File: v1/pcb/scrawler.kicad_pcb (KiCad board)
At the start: 2 copper layers, 185.3 x 172.6 mm, 97 parts, among them J2 MJ-4PP-9, J3 OLED, SW10A1 SW_PUSH, SW10B1 SW_PUSH, SW11A1 SW_PUSH, SW11B1 SW_PUSH, SW12A1 SW_PUSH, SW12B1 SW_PUSH, SW13A1 SW_PUSH, SW13B1 SW_PUSH, SW14A1 SW_PUSH, SW14B1 SW_PUSH, SW15A1 SW_PUSH, SW15B1 SW_PUSH, SW16A1 SW_PUSH, SW16B1 SW_PUSH, SW17A1 SW_PUSH, SW17B1 SW_PUSH, SW18A1 SW_PUSH, SW18B1 SW_PUSH, SW19A1 SW_PUSH, SW19B1 SW_PUSH, SW1A1 SW_PUSH, SW1B1 SW_PUSH, SW20A1 SW_PUSH, SW20B1 SW_PUSH, SW21A1 SW_PUSH, SW21B1 SW_PUSH, SW22A1 SW_PUSH, SW22B1 SW_PUSH, SW24A1 SW_PUSH, SW24B1 SW_PUSH, SW25A1 SW_PUSH, SW25B1 SW_PUSH, SW26 Rotary_Encoder_Switch, SW26A1 SW_PUSH, SW26B1 SW_PUSH, SW2A1 SW_PUSH, SW2B1 SW_PUSH, SW3A1 SW_PUSH, SW3B1 SW_PUSH, SW4A1 SW_PUSH, SW4B1 SW_PUSH, SW5A1 SW_PUSH, SW5B1 SW_PUSH, SW6A1 SW_PUSH, SW6B1 SW_PUSH, SW7A1 SW_PUSH, SW7B1 SW_PUSH, SW8A1 SW_PUSH, SW8B1 SW_PUSH, SW9A1 SW_PUSH, SW9B1 SW_PUSH, U1 ProMicro

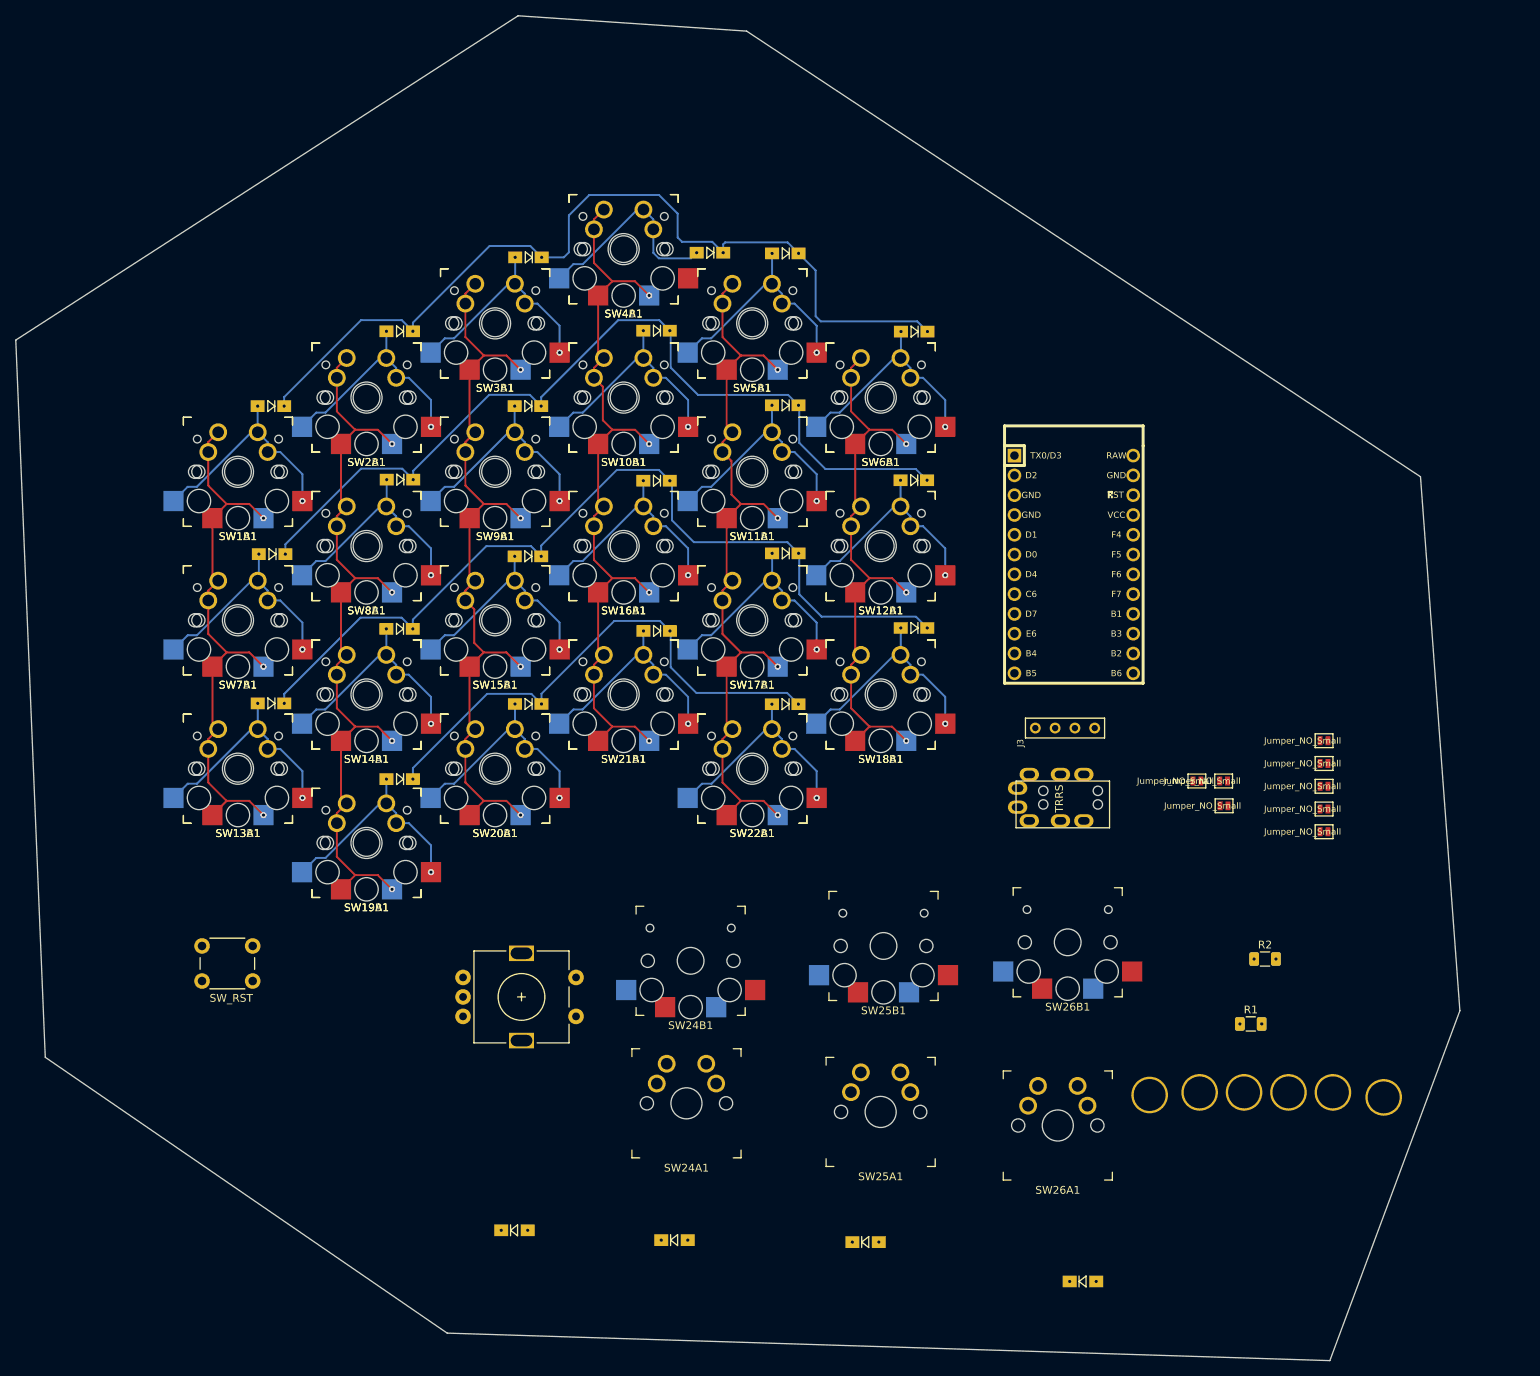
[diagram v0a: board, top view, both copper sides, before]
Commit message: pcb done
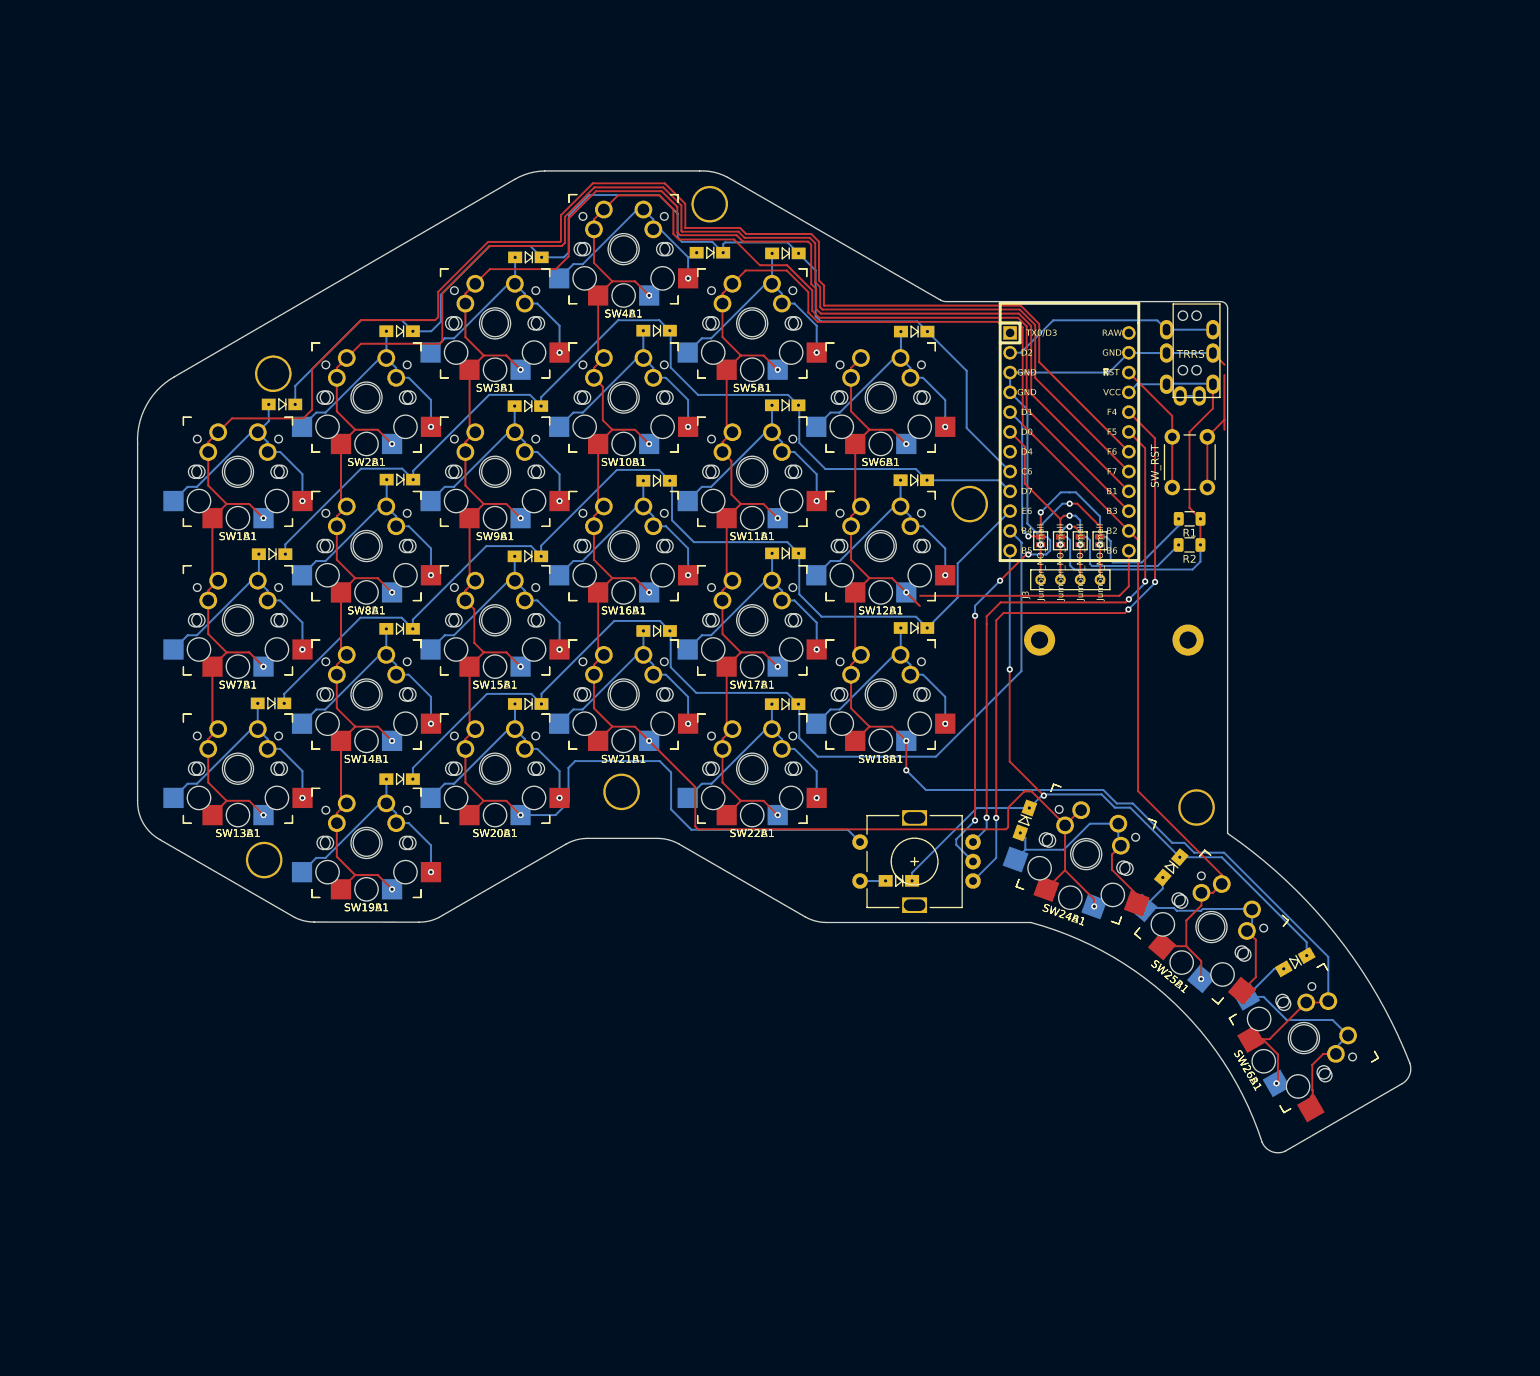
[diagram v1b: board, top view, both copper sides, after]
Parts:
- added H7: Hole, SofleKeyboard-footprint:M2_HOLE_PCB, F.Cu at (179.1, 97.8)
- added H8: Hole, SofleKeyboard-footprint:M2_HOLE_PCB, F.Cu at (198.1, 97.8)
- JP5, JP6, JP7, JP8: moved to B.Cu
- moved H1 145.6 mm to (80.7, 63.6)
- moved RSW1 144.6 mm to (200.6, 71.7), turned to 270 degrees
- moved H6 143.6 mm to (136.7, 41.9)
- moved H2 123.7 mm to (79.6, 126.0)
- moved H5 88.7 mm to (170.1, 80.3)
- moved H3 88.7 mm to (125.4, 117.3)
- moved D24 70.1 mm to (177.2, 120.9), turned to 250 degrees
- moved D23 66.7 mm to (161.0, 128.7), turned to 180 degrees
- moved R1 65.3 mm to (198.3, 82.2), turned to 180 degrees
- moved J2 65.2 mm to (199.2, 54.7), turned to 0 degrees
- moved D25 62.1 mm to (196.0, 127.0), turned to 230 degrees
- moved SW24A1 60.4 mm to (185.1, 125.3), turned to 340 degrees
- moved R2 54.0 mm to (198.3, 85.6), turned to 180 degrees
- moved SW26 53.4 mm to (163.0, 126.2), turned to 180 degrees
- moved SW24B1 52.6 mm to (185.1, 125.3), turned to 340 degrees
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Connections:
- SW24A1 pad 1: COL1 -> COL3
- SW24B1 pad 1: COL1 -> COL3
- SW25A1 pad 1: COL2 -> COL4
- SW25B1 pad 1: COL2 -> COL4
- SW26 pad S1: COL0 -> COL2
- SW26A1 pad 1: COL3 -> COL5
- SW26B1 pad 1: COL3 -> COL5
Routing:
- net COL3: track 100.1 -> 279.2 mm, vias 4 -> 5
- net COL2: track 100.1 -> 275.2 mm
- net COL0: track 75.5 -> 235.9 mm
- net COL4: track 100.1 -> 243.4 mm, vias 4 -> 5
- net COL1: track 102.8 -> 243.2 mm
- net GND: track 0.00 -> 131.5 mm, vias 0 -> 5
- net COL5: track 73.0 -> 199.3 mm, vias 3 -> 5
- net ROW4: track 0.00 -> 98.9 mm, vias 0 -> 2
- net ENCA: track 0.00 -> 80.4 mm, vias 0 -> 3
- net ENCB: track 0.00 -> 72.1 mm, vias 0 -> 3
- net VCC: track 0.00 -> 62.2 mm, vias 0 -> 1
- net ROW3: track 67.6 -> 124.7 mm
- net SDA: track 0.00 -> 49.9 mm, vias 0 -> 2
- net SCL: track 0.00 -> 38.8 mm, vias 0 -> 1
- net Net-(D26-Pad2): track 0.00 -> 33.7 mm
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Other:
- board size 185.3 x 172.6 mm -> 163.4 x 126 mm

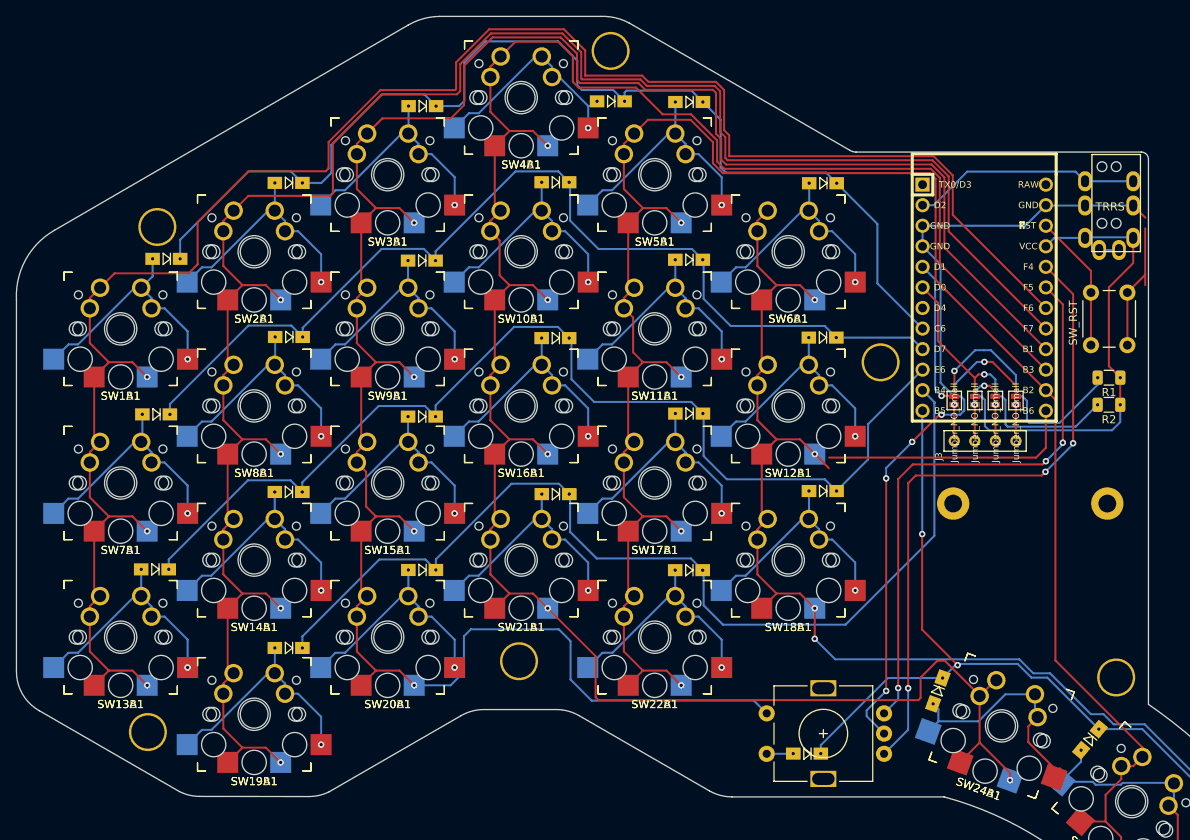
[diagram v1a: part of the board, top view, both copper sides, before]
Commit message: pcb plate finished
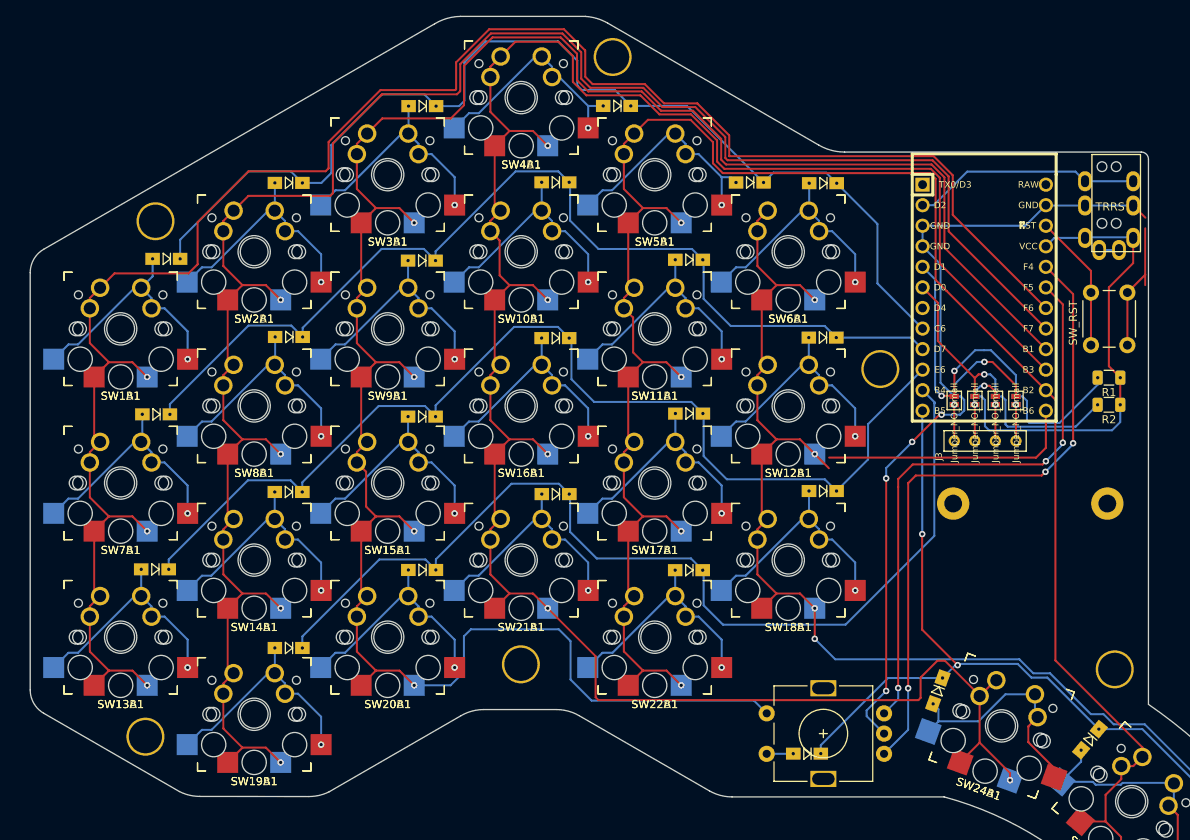
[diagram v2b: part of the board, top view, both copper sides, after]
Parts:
- moved D5 12.5 mm to (153.9, 58.1)
- moved H4 1.02 mm to (199.0, 118.3)
- moved D4 0.95 mm to (137.5, 48.7)
- moved H5 0.83 mm to (170.1, 81.2)
- moved H6 0.79 mm to (137.0, 42.6)
- moved H1 0.75 mm to (80.5, 62.9)
- moved H2 0.65 mm to (79.3, 126.6)
- moved H3 0.44 mm to (125.7, 117.7)
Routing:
- net ROW0: track 137.4 -> 133.3 mm
- net COL2: track 275.2 -> 272.3 mm
- net COL1: track 243.2 -> 240.3 mm
- net COL0: track 235.9 -> 233.0 mm
- net Net-(D5-Pad2): track 30.9 -> 29.0 mm
- net Net-(D4-Pad2): track 27.5 -> 28.1 mm
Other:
- board size 163.4 x 126 mm -> 161.7 x 126 mm
